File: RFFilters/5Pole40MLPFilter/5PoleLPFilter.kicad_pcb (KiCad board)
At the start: 2 copper layers, 38.1 x 12.7 mm, 7 parts, among them J1 FilterConn02

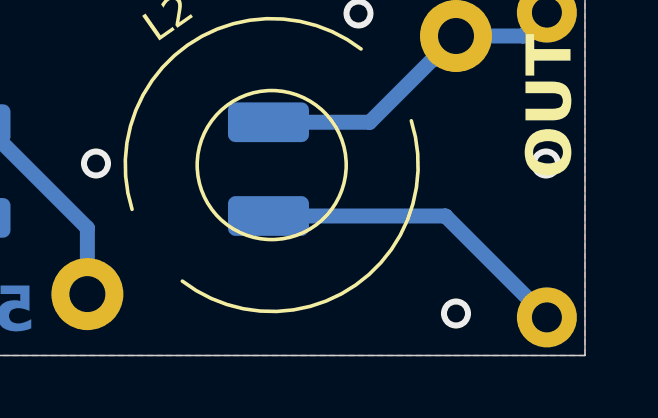
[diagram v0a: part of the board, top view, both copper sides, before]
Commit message: Update 5PoleLP Filter
+ V4.00 Hardware LP Filter PCB
+ Remove deprecated files
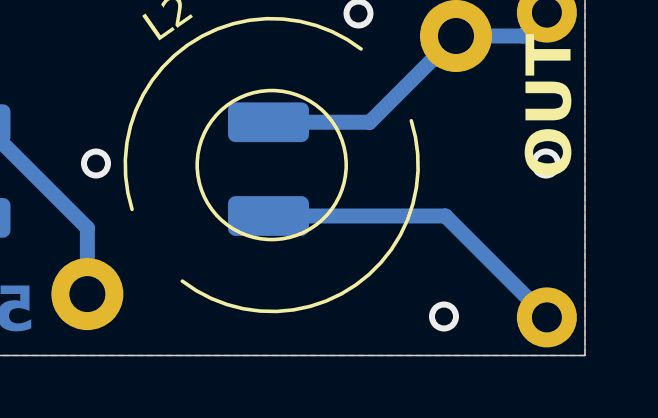
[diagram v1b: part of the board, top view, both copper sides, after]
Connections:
- net Net-(C2-Pad1) renamed /Mid
- C1 pad 1: Net-(C1-Pad1) -> (no net)
- C3 pad 1: Net-(C3-Pad1) -> (no net)
- L1 pad 1: Net-(C1-Pad1) -> (no net)
- L2 pad 2: Net-(C3-Pad1) -> (no net)
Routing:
- net Net-(C1-Pad1): track 9.75 -> 0.00 mm
- net IN: track 9.48 -> 19.2 mm
- net OUT: track 3.40 -> 11.3 mm
- net Net-(C3-Pad1): track 7.94 -> 0.00 mm
